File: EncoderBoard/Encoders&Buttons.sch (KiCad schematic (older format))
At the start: 75 parts, among them SW1 Rotary_Encoder_Switch, SW10 SW_Push_LED_Red, SW11 SW_Push_LED_Blue, SW12 SW_Push_LED_Red, SW13 SW_Push_LED_Yellow, SW14 SW_Push_LED_Green, SW15 SW_Push_LED_Blue, SW2 Rotary_Encoder_Switch, SW3 Rotary_Encoder_Switch, SW4 Rotary_Encoder_Switch, SW5 Rotary_Encoder_Switch, SW6 Rotary_Encoder_Switch, SW7 Rotary_Encoder_Switch, SW8 Rotary_Encoder_Switch, SW9 Rotary_Encoder_Switch

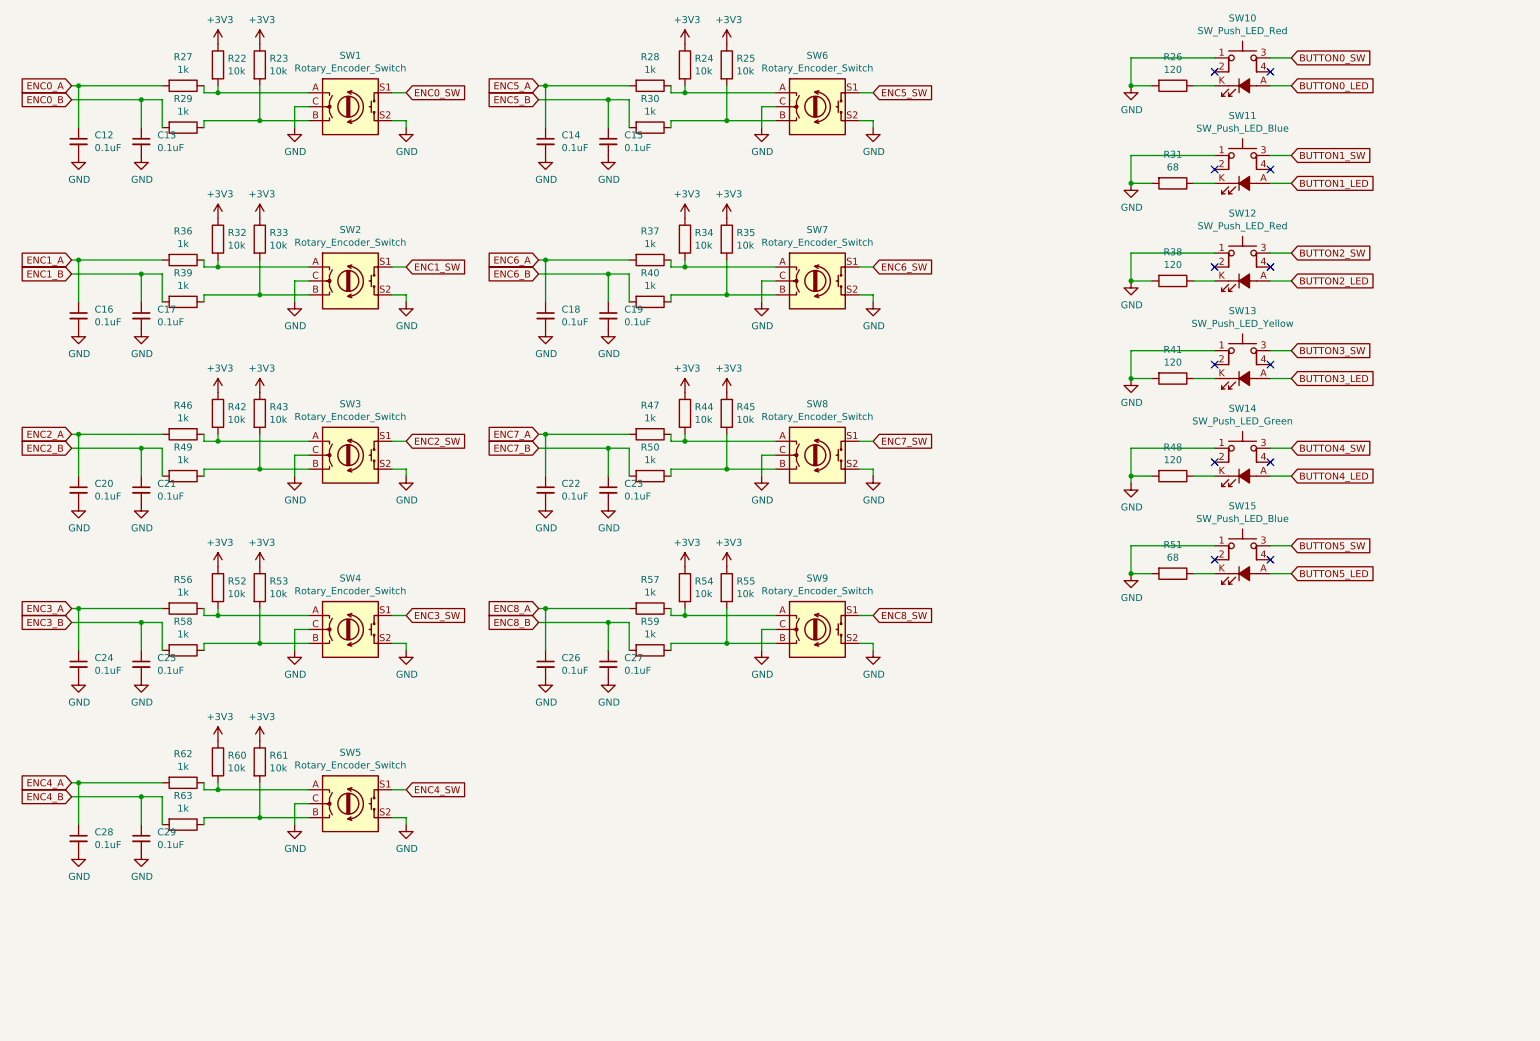
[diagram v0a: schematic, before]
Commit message: Tidied up the encoder board, updated debounce logic for schematic.
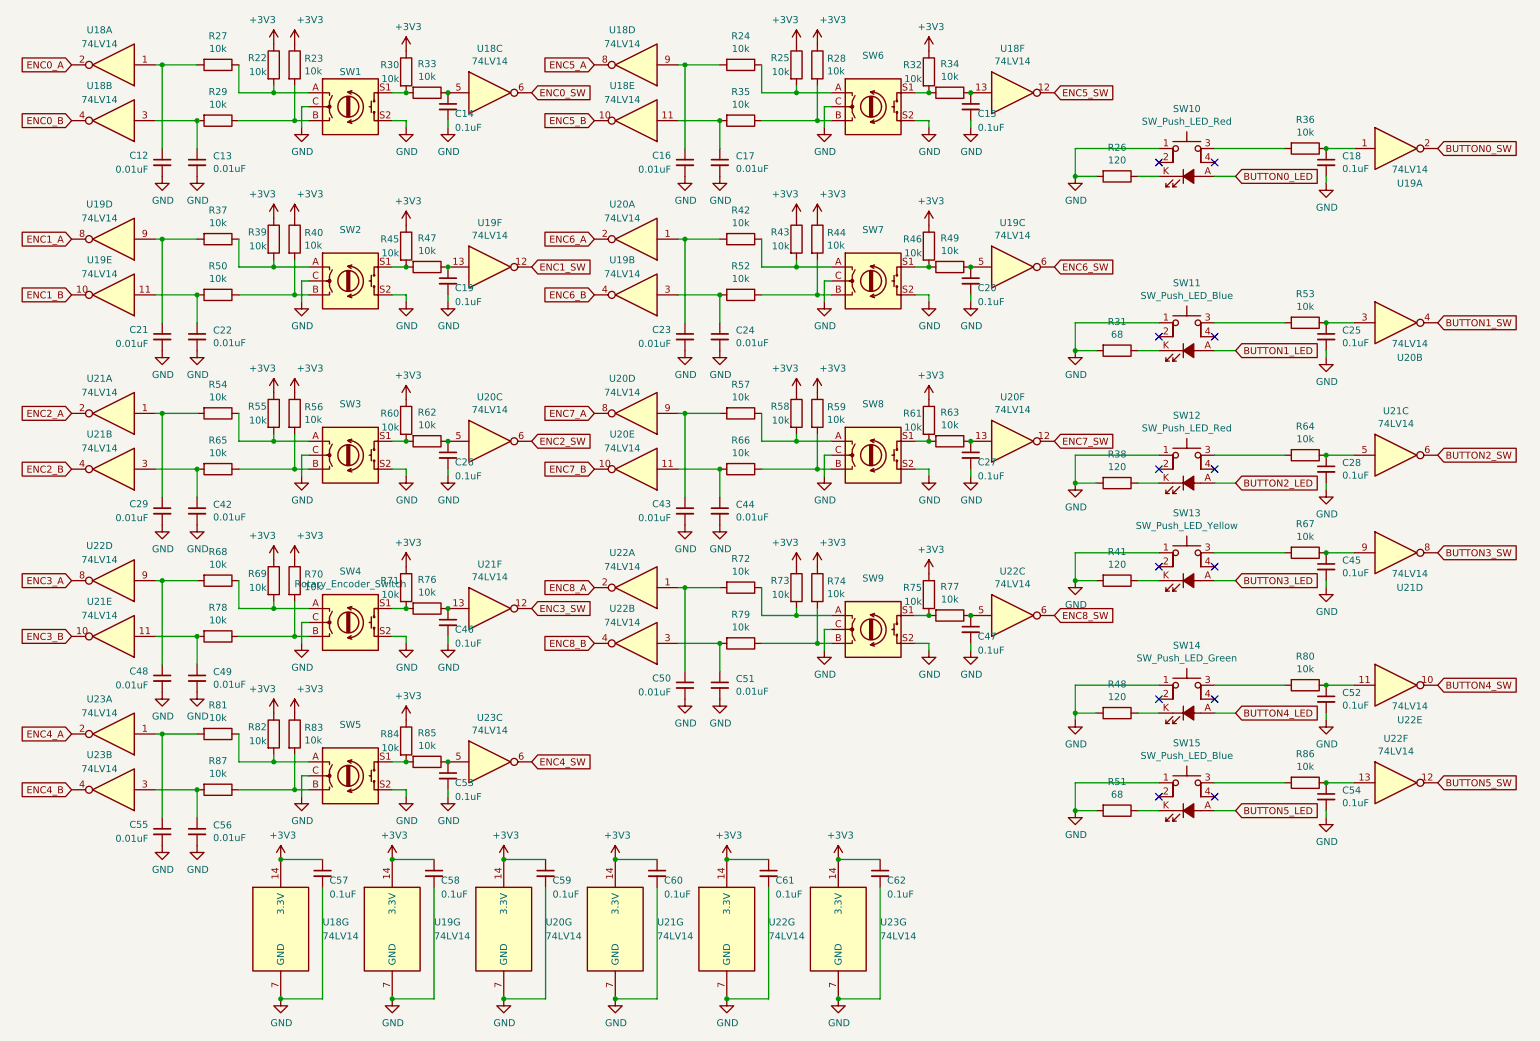
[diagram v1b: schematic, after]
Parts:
- added C42, C43, C44, C48, C49, C50, C51, C55, C56: 0.01uF, Capacitor_BG:C_0805_2012Metric, symbol Device:C_Small
- added C45, C46, C47, C52, C53, C54, C57, C58, C59, C60, C61, C62: 0.1uF, Capacitor_BG:C_0805_2012Metric, symbol Device:C_Small
- added R64, R65, R66, R67, R68, R69, R70, R71, R72, R73, R74, R75, R76, R77, R78, R79, R80, R81, R82, R83, R84, R85, R86, R87: 10k, Resistor_BG:R_0805_2012Metric, symbol Device:R
- added U18, U19, U20, U21, U22, U23: 74LV14, symbol 74xx:74LV14
- C12, C13, C16, C17, C21, C22, C23, C24, C29: value 0.1uF -> 0.01uF
- R27, R28, R29, R30, R36, R37, R39, R40, R46, R47, R49, R50, R56, R57, R58, R59, R62, R63: value 1k -> 10k
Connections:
- net +3V3: now also R28.1, R30.1, R39.1, R40.1, R46.1, R56.1, R58.1, R59.1, C57.1, C58.1, C59.1, C60.1, C61.1, C62.1, R69.1, R70.1, R71.1, R73.1, R74.1, R75.1, R82.1, R83.1, R84.1, U18.14 (3.3V), U19.14 (3.3V), U20.14 (3.3V), U21.14 (3.3V), U22.14 (3.3V), U23.14 (3.3V); no longer R24.1, R33.1, R34.1, R35.1, R42.1, R52.1, R53.1, R54.1
- net BUTTON0_SW: now also U19.2; no longer SW10.3
- net BUTTON1_SW: now also U20.4; no longer SW11.3
- net BUTTON2_SW: now also U21.6; no longer SW12.3
- net BUTTON3_SW: now also U21.8; no longer SW13.3
- net BUTTON4_SW: now also U22.10; no longer SW14.3
- net BUTTON5_SW: now also U22.12; no longer SW15.3
- net ENC0_A: now also U18.2; no longer C12.1, R27.2
- net ENC0_B: now also U18.4; no longer C13.1, R29.2
- net ENC0_SW: now also U18.6; no longer SW1.S1
- net ENC1_A: now also U19.8; no longer C16.1, R36.2
- net ENC1_B: now also U19.10; no longer C17.1, R39.2
- net ENC1_SW: now also U19.12; no longer SW2.S1
- net ENC2_A: now also U21.2; no longer C20.1, R46.2
- net ENC2_B: now also U21.4; no longer C21.1, R49.2
- net ENC2_SW: now also U20.6; no longer SW3.S1
- net ENC3_A: now also U22.8; no longer C24.1, R56.2
- net ENC3_B: now also U21.10; no longer C25.1, R58.2
- net ENC3_SW: now also U21.12; no longer SW4.S1
- net ENC4_A: now also U23.2; no longer C28.1, R62.2
- net ENC4_B: now also U23.4; no longer C29.1, R63.2
- net ENC4_SW: now also U23.6; no longer SW5.S1
- net ENC5_A: now also U18.8; no longer C14.1, R28.2
- net ENC5_B: now also U18.10; no longer C15.1, R30.2
- net ENC5_SW: now also U18.12; no longer SW6.S1
- net ENC6_A: now also U20.2; no longer C18.1, R37.2
- net ENC6_B: now also U19.4; no longer C19.1, R40.2
- net ENC6_SW: now also U19.6; no longer SW7.S1
- net ENC7_A: now also U20.8; no longer C22.1, R47.2
- net ENC7_B: now also U20.10; no longer C23.1, R50.2
- net ENC7_SW: now also U20.12; no longer SW8.S1
- net ENC8_A: now also U22.2; no longer C26.1, R57.2
- net ENC8_B: now also U22.4; no longer C27.1, R59.2
- net ENC8_SW: now also U22.6; no longer SW9.S1
- net GND: now also C42.2, C43.2, C44.2, C45.2, C46.2, C47.2, C48.2, C49.2, C50.2, C51.2, C52.2, C53.2, C54.2, C55.2, C56.2, C57.2, C58.2, C59.2, C60.2, C61.2, C62.2, U18.7 (GND), U19.7 (GND), U20.7 (GND), U21.7 (GND), U22.7 (GND), U23.7 (GND)
- new net: R53.2, SW11.3
- new net: R36.2, SW10.3
- new net: R30.2, R33.2, SW1.S1
- new net: C12.1, R27.2, U18.1
- new net: C13.1, R29.2, U18.3
- new net: R37.1, R39.2, SW2.A
- new net: R40.2, R50.1, SW2.B
- new net: R45.2, R47.2, SW2.S1
- new net: R54.1, R55.2, SW3.A
- new net: R56.2, R65.1, SW3.B
- new net: R60.2, R62.2, SW3.S1
- new net: R68.1, R69.2, SW4.A
- new net: R70.2, R78.1, SW4.B
- new net: R71.2, R76.2, SW4.S1
- new net: R81.1, R82.2, SW5.A
- new net: R83.2, R87.1, SW5.B
- new net: R84.2, R85.2, SW5.S1
- new net: R24.1, R25.2, SW6.A
- new net: R28.2, R35.1, SW6.B
- new net: R32.2, R34.2, SW6.S1
- new net: R42.1, R43.2, SW7.A
- new net: R44.2, R52.1, SW7.B
- new net: R46.2, R49.2, SW7.S1
- new net: R57.1, R58.2, SW8.A
- new net: R59.2, R66.1, SW8.B
- new net: R61.2, R63.2, SW8.S1
- new net: R72.1, R73.2, SW9.A
- new net: R74.2, R79.1, SW9.B
- new net: R75.2, R77.2, SW9.S1
- new net: R64.2, SW12.3
- new net: R67.2, SW13.3
- new net: R80.2, SW14.3
- new net: R86.2, SW15.3
- new net: C14.1, R33.1, U18.5
- new net: C18.1, R36.1, U19.1
- new net: C25.1, R53.1, U20.3
- new net: C28.1, R64.1, U21.5
- new net: C45.1, R67.1, U21.9
- new net: C52.1, R80.1, U22.11
- new net: C54.1, R86.1, U22.13
- new net: C21.1, R37.2, U19.9
- new net: C22.1, R50.2, U19.11
- new net: C19.1, R47.1, U19.13
- new net: C29.1, R54.2, U21.1
- new net: C42.1, R65.2, U21.3
- new net: C48.1, R68.2, U22.9
- new net: C49.1, R78.2, U21.11
- new net: C55.1, R81.2, U23.1
- new net: C56.1, R87.2, U23.3
- new net: C16.1, R24.2, U18.9
- new net: C17.1, R35.2, U18.11
- new net: C26.1, R62.1, U20.5
- new net: C46.1, R76.1, U21.13
- new net: C53.1, R85.1, U23.5
- new net: C15.1, R34.1, U18.13
- new net: C23.1, R42.2, U20.1
- new net: C24.1, R52.2, U19.3
- new net: C43.1, R57.2, U20.9
- new net: C44.1, R66.2, U20.11
- new net: C50.1, R72.2, U22.1
- new net: C51.1, R79.2, U22.3
- new net: C20.1, R49.1, U19.5
- new net: C27.1, R63.1, U20.13
- new net: C47.1, R77.1, U22.5
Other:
- moved on the sheet: C12, C13, R22, R23, R26, R27, R29, R31, R38, R41, R48, R51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
